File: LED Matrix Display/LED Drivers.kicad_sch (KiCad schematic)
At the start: 8 parts, among them U1 MAX7219, U2 MAX7219, U3 MAX7219, U4 MAX7219, U5 KWM-R30881CBB, U6 KWM-R30881CBB, U7 KWM-R30881CBB, U8 KWM-R30881CBB

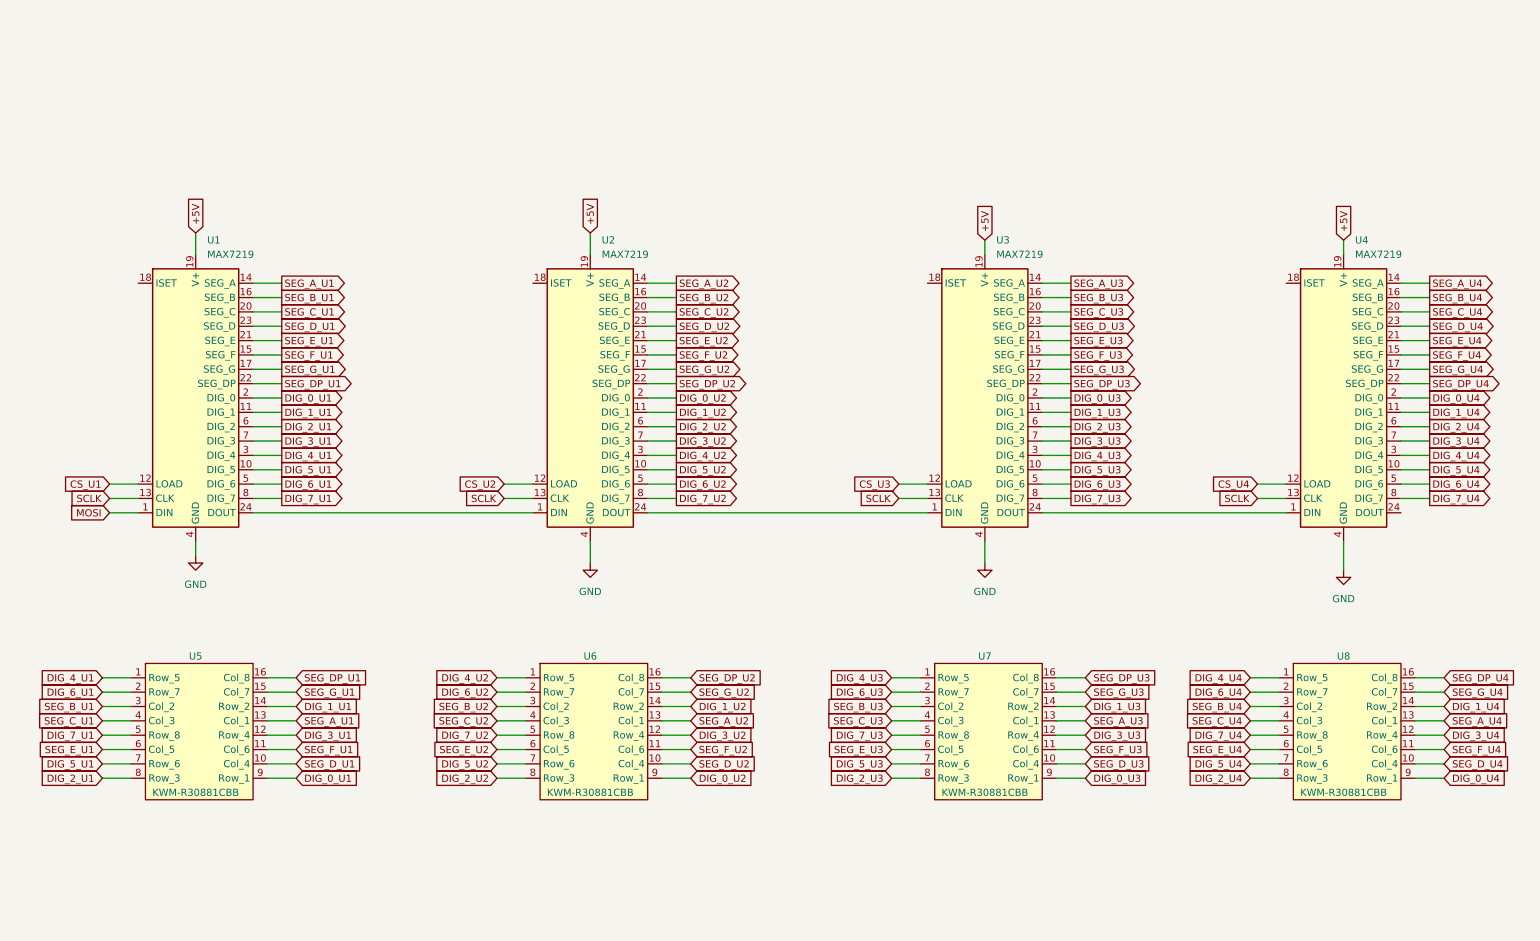
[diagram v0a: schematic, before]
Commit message: SCH and PCB updates
Added updates to SCH and made progress on layout.
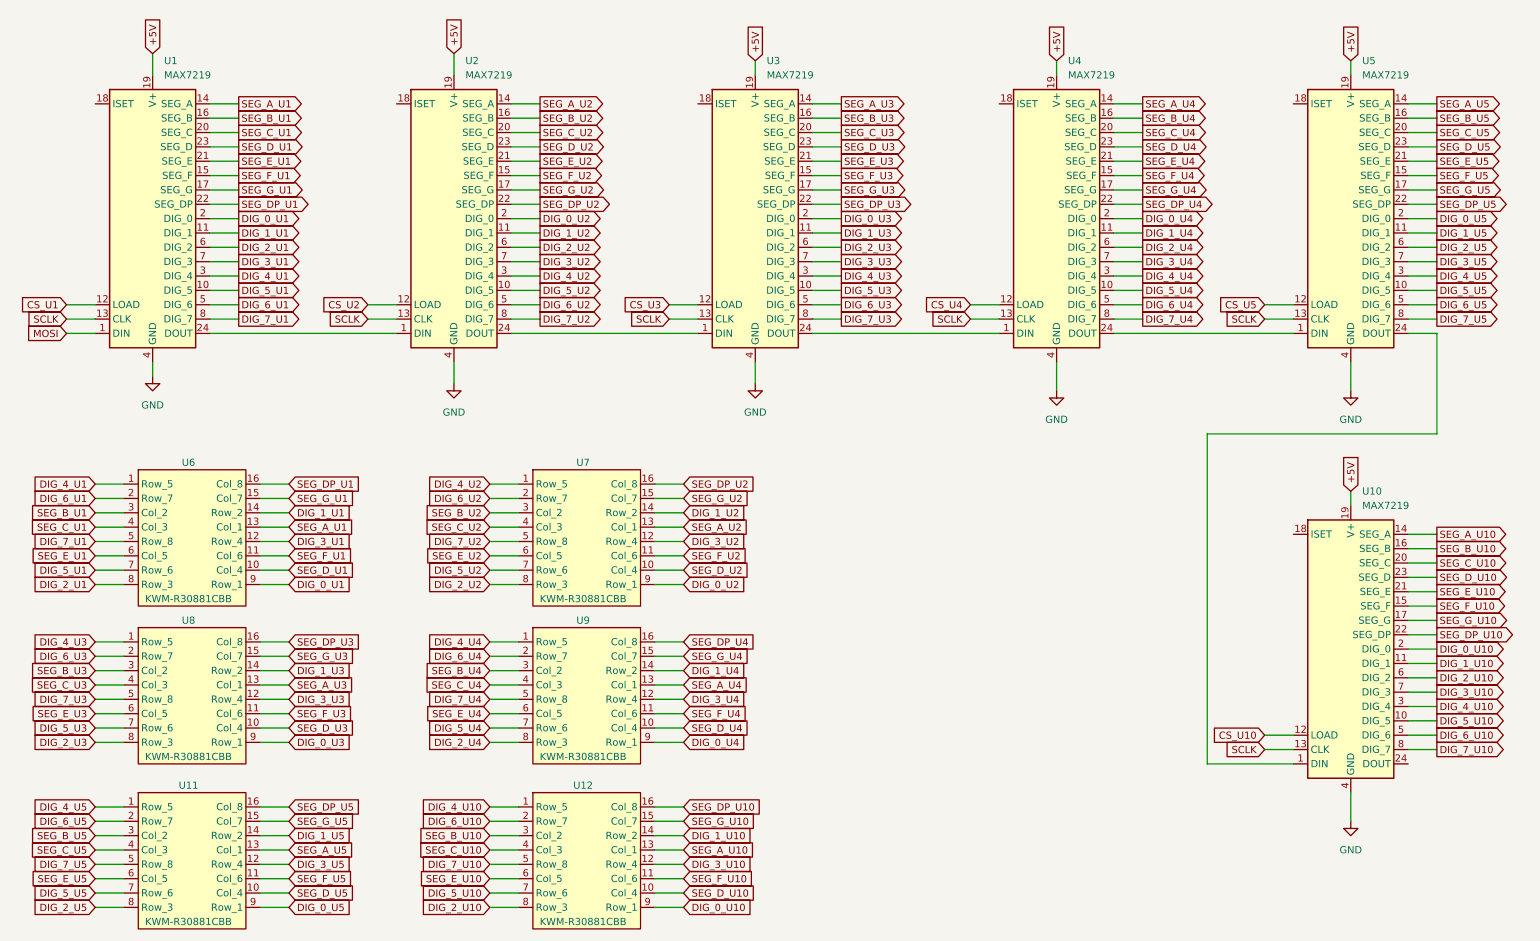
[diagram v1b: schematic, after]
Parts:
- added U10, U5: MAX7219, Package_SO:SOIC-24W_7.5x15.4mm_P1.27mm, symbol Driver_LED:MAX7219
- added U11, U12: KWM-R30881CBB, 1_My_Custom_Library:KWM-R30881CBB, symbol Display_LED:KWM-R30881CBB
- U1: footprint (none) -> Package_SO:SOIC-24W_7.5x15.4mm_P1.27mm
- U6: renamed from U5; footprint (none) -> 1_My_Custom_Library:KWM-R30881CBB
- U7: renamed from U6; footprint (none) -> 1_My_Custom_Library:KWM-R30881CBB
- U8: renamed from U7; footprint (none) -> 1_My_Custom_Library:KWM-R30881CBB
- U9: renamed from U8; footprint (none) -> 1_My_Custom_Library:KWM-R30881CBB
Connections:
- net +5V: now also U10.19 (V+), U5.19 (V+)
- net GND: now also U10.4 (GND), U10.9 (GND), U5.4 (GND), U5.9 (GND)
- net SCLK: now also U10.13 (CLK), U5.13 (CLK)
- net at U4.24 (DOUT): now also U5.1 (DIN)
- new net: U10.1 (DIN), U5.24 (DOUT)
- new net CS_U10: U10.12 (LOAD)
- new net CS_U5: U5.12 (LOAD)
- new net DIG_0_U10: U10.2 (DIG_0), U12.9 (Row_1)
- new net DIG_0_U5: U11.9 (Row_1), U5.2 (DIG_0)
- new net DIG_1_U10: U10.11 (DIG_1), U12.14 (Row_2)
- new net DIG_1_U5: U11.14 (Row_2), U5.11 (DIG_1)
- new net DIG_2_U10: U10.6 (DIG_2), U12.8 (Row_3)
- new net DIG_2_U5: U11.8 (Row_3), U5.6 (DIG_2)
- new net DIG_3_U10: U10.7 (DIG_3), U12.12 (Row_4)
- new net DIG_3_U5: U11.12 (Row_4), U5.7 (DIG_3)
- new net DIG_4_U10: U10.3 (DIG_4), U12.1 (Row_5)
- new net DIG_4_U5: U11.1 (Row_5), U5.3 (DIG_4)
- new net DIG_5_U10: U10.10 (DIG_5), U12.7 (Row_6)
- new net DIG_5_U5: U11.7 (Row_6), U5.10 (DIG_5)
- new net DIG_6_U10: U10.5 (DIG_6), U12.2 (Row_7)
- new net DIG_6_U5: U11.2 (Row_7), U5.5 (DIG_6)
- new net DIG_7_U10: U10.8 (DIG_7), U12.5 (Row_8)
- new net DIG_7_U5: U11.5 (Row_8), U5.8 (DIG_7)
- new net SEG_A_U10: U10.14 (SEG_A), U12.13 (Col_1)
- new net SEG_A_U5: U11.13 (Col_1), U5.14 (SEG_A)
- new net SEG_B_U10: U10.16 (SEG_B), U12.3 (Col_2)
- new net SEG_B_U5: U11.3 (Col_2), U5.16 (SEG_B)
- new net SEG_C_U10: U10.20 (SEG_C), U12.4 (Col_3)
- new net SEG_C_U5: U11.4 (Col_3), U5.20 (SEG_C)
- new net SEG_DP_U10: U10.22 (SEG_DP), U12.16 (Col_8)
- new net SEG_DP_U5: U11.16 (Col_8), U5.22 (SEG_DP)
- new net SEG_D_U10: U10.23 (SEG_D), U12.10 (Col_4)
- new net SEG_D_U5: U11.10 (Col_4), U5.23 (SEG_D)
- new net SEG_E_U10: U10.21 (SEG_E), U12.6 (Col_5)
- new net SEG_E_U5: U11.6 (Col_5), U5.21 (SEG_E)
- new net SEG_F_U10: U10.15 (SEG_F), U12.11 (Col_6)
- new net SEG_F_U5: U11.11 (Col_6), U5.15 (SEG_F)
- new net SEG_G_U10: U10.17 (SEG_G), U12.15 (Col_7)
- new net SEG_G_U5: U11.15 (Col_7), U5.17 (SEG_G)
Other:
- moved on the sheet: U1, U2, U3, U4, U6, U7, U8, U9
